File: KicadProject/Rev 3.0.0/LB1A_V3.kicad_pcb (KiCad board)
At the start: 6 copper layers, 45 x 45 mm, 188 parts, among them J601 2337019-1, J602 2337019-1, U101 STM32MP157CAA3, U201 AS4C256M16D3LC-12BCN, U401 STPMIC1xPQR, U501 S40FC004C1B2C00000, U601 LBEE59B1LV-278, U701 DF40C-70DP-0.4V(51), U702 DF40C-100DP-0.4V(51), U703 DF40C-100DP-0.4V(51), X101 32.768kHz, Y101 24MHz

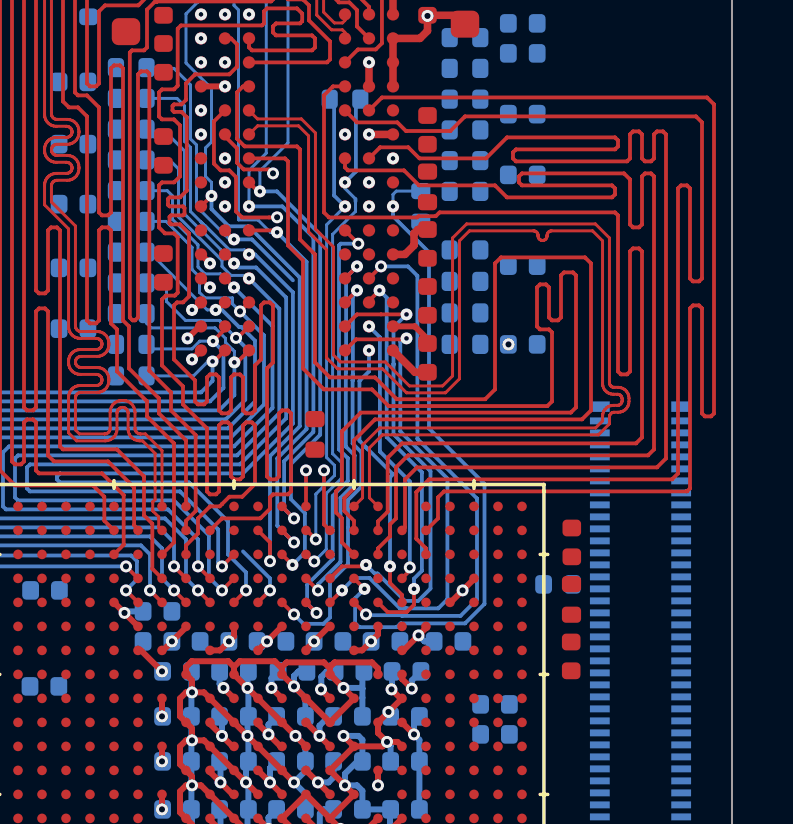
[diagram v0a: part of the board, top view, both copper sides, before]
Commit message: little more done
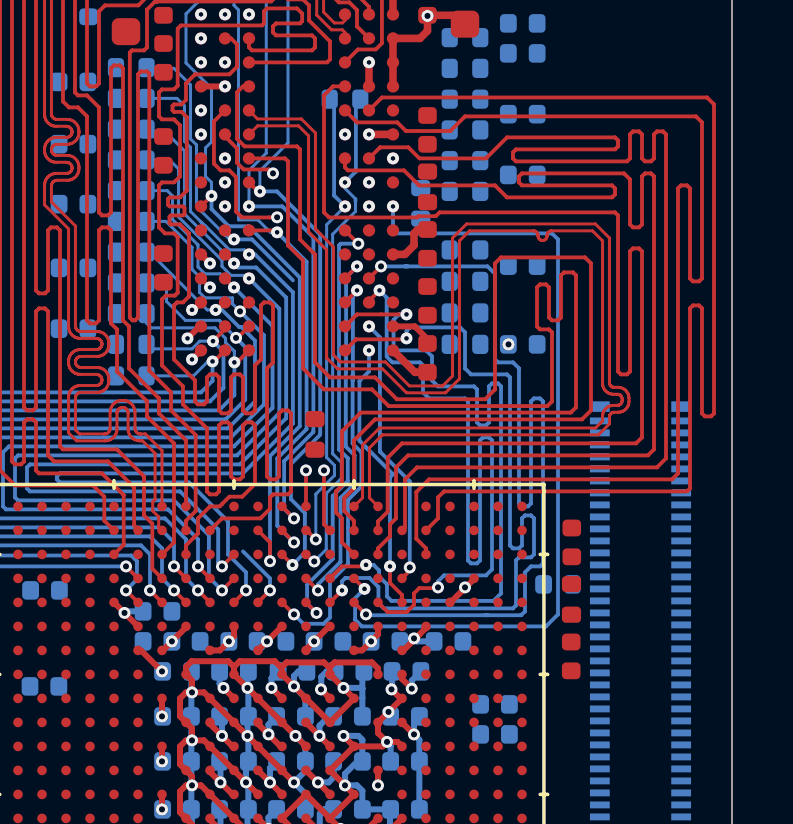
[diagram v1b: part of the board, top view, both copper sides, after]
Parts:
- moved R222 0.10 mm to (134.6, 95.2)
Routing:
- net /MPU_DDR3L_Memory/DDR_A4: track 13.2 -> 26.1 mm
- net /MPU_DDR3L_Memory/DDR_BA1: track 18.0 -> 30.7 mm
- net /MPU_DDR3L_Memory/DDR_A14: track 16.6 -> 25.8 mm
- net /MPU_DDR3L_Memory/DDR_A11: track 16.3 -> 24.5 mm
- net /MPU_DDR3L_Memory/DDR_CKE: track 22.4 -> 27.6 mm
